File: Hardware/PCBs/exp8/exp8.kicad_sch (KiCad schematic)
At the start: 5 parts, among them J1 Conn_01x07_Female, J2 Conn_01x02_Female, U1 7410, U2 7410, U3 7400

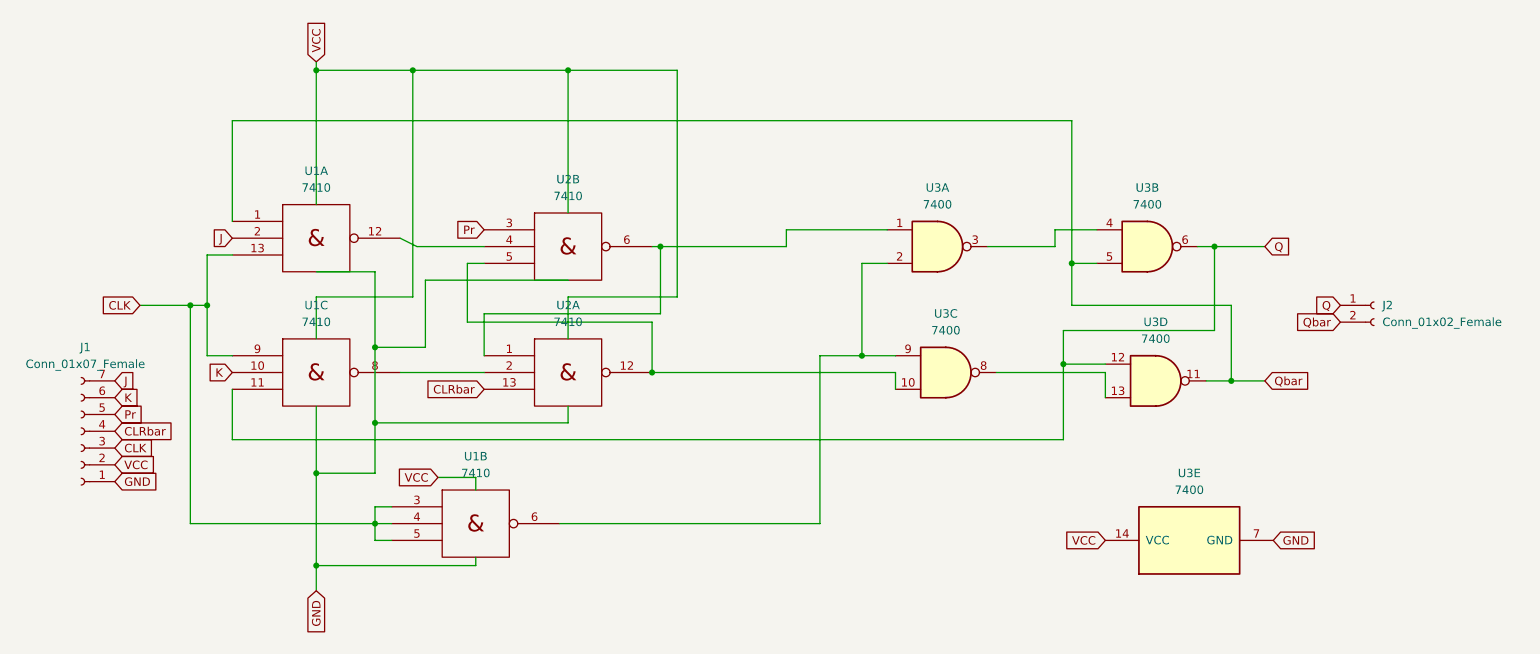
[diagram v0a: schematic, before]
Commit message: Multiple PCBs updated
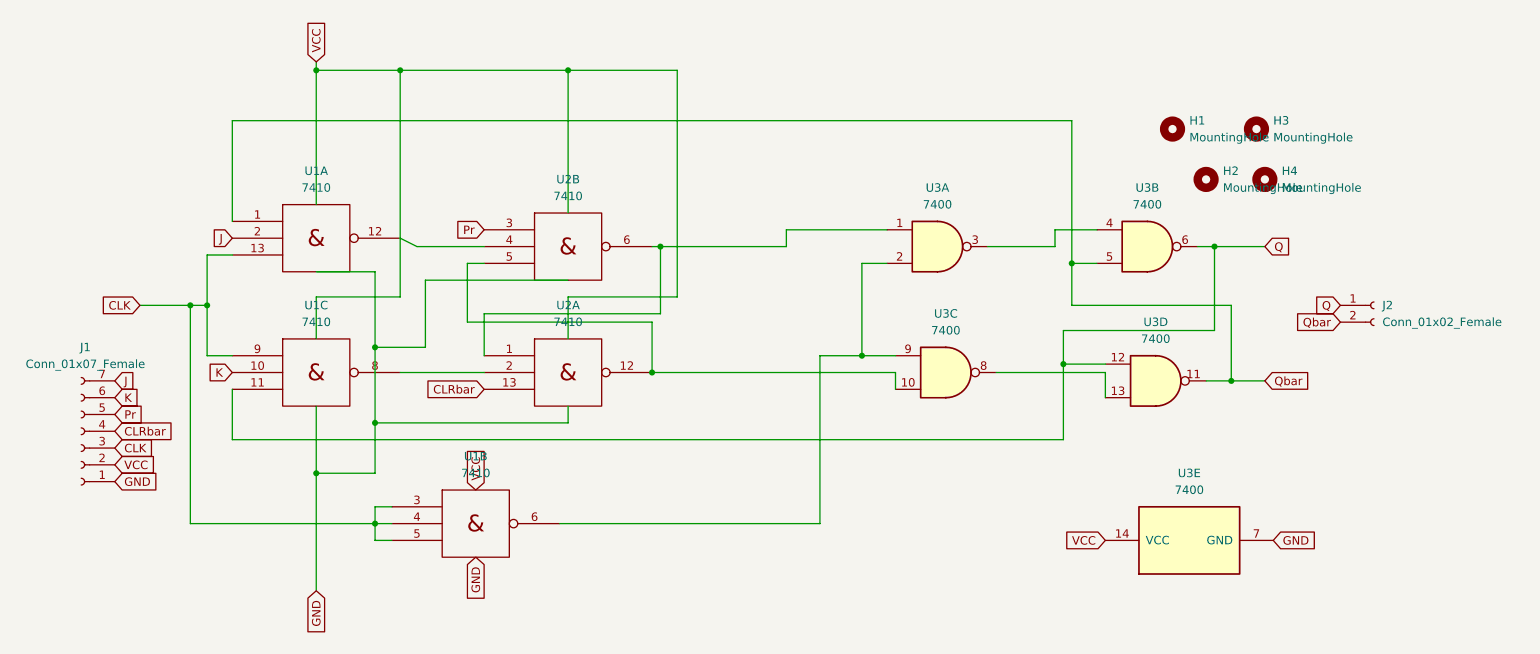
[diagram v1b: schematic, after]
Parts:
- added H1, H2, H3, H4: MountingHole, MountingHole:MountingHole_2.5mm, symbol Mechanical:MountingHole
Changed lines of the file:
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@@
   (junction (at 57.15 21.59) (diameter 0) (color 0 0 0 0)
   )
-  (junction (at 71.755 21.59) (diameter 0) (color 0 0 0 0)
-  )
   (junction (at 40.64 57.15) (diameter 0) (color 0 0 0 0)
   )
@@
   (junction (at 139.7 64.77) (diameter 0) (color 0 0 0 0)
   )
-  (junction (at 57.15 96.52) (diameter 0) (color 0 0 0 0)
-  )
   (junction (at 107.95 67.31) (diameter 0) (color 0 0 0 0)
   )
   (junction (at 171.45 50.8) (diameter 0) (color 0 0 0 0)
   )
+  (junction (at 69.85 21.59) (diameter 0) (color 0 0 0 0)
+  )
   (junction (at 95.25 21.59) (diameter 0) (color 0 0 0 0)
   )
@@
     (stroke (width 0) (type default) (color 0 0 0 0))
   )
-  (wire (pts (xy 57.15 21.59) (xy 71.755 21.59))
-    (stroke (width 0) (type default) (color 0 0 0 0))
-  )
   (wire (pts (xy 95.25 72.39) (xy 95.25 74.93))
     (stroke (width 0) (type default) (color 0 0 0 0))
@@
     (stroke (width 0) (type default) (color 0 0 0 0))
   )
-  (wire (pts (xy 95.25 21.59) (xy 71.755 21.59))
-    (stroke (width 0) (type default) (color 0 0 0 0))
-  )
-  (wire (pts (xy 57.15 55.88) (xy 71.755 55.88))
+  (wire (pts (xy 95.25 21.59) (xy 69.85 21.59))
+    (stroke (width 0) (type default) (color 0 0 0 0))
+  )
+  (wire (pts (xy 57.15 55.88) (xy 69.85 55.88))
     (stroke (width 0) (type default) (color 0 0 0 0))
   )
@@
     (stroke (width 0) (type default) (color 0 0 0 0))
   )
-  (wire (pts (xy 75.565 83.185) (xy 81.28 83.185))
-    (stroke (width 0) (type default) (color 0 0 0 0))
-  )
   (wire (pts (xy 168.91 48.26) (xy 168.91 45.72))
     (stroke (width 0) (type default) (color 0 0 0 0))
@@
     (stroke (width 0) (type default) (color 0 0 0 0))
   )
-  (wire (pts (xy 57.15 82.55) (xy 57.15 96.52))
+  (wire (pts (xy 57.15 82.55) (xy 57.15 100.33))
     (stroke (width 0) (type default) (color 0 0 0 0))
   )
@@
     (stroke (width 0) (type default) (color 0 0 0 0))
   )
-  (wire (pts (xy 57.15 96.52) (xy 57.15 100.33))
-    (stroke (width 0) (type default) (color 0 0 0 0))
-  )
   (wire (pts (xy 109.22 48.26) (xy 128.27 48.26))
     (stroke (width 0) (type default) (color 0 0 0 0))
@@
     (stroke (width 0) (type default) (color 0 0 0 0))
   )
-  (wire (pts (xy 71.755 21.59) (xy 71.755 55.88))
+  (wire (pts (xy 69.85 21.59) (xy 69.85 55.88))
     (stroke (width 0) (type default) (color 0 0 0 0))
   )
@@
     (stroke (width 0) (type default) (color 0 0 0 0))
   )
-  (wire (pts (xy 81.28 95.25) (xy 81.28 96.52))
-    (stroke (width 0) (type default) (color 0 0 0 0))
-  )
   (wire (pts (xy 66.04 74.93) (xy 66.04 82.55))
     (stroke (width 0) (type default) (color 0 0 0 0))
@@
     (stroke (width 0) (type default) (color 0 0 0 0))
   )
-  (wire (pts (xy 81.28 83.185) (xy 81.28 85.09))
-    (stroke (width 0) (type default) (color 0 0 0 0))
-  )
   (wire (pts (xy 66.04 87.63) (xy 66.04 90.17))
     (stroke (width 0) (type default) (color 0 0 0 0))
@@
     (stroke (width 0) (type default) (color 0 0 0 0))
   )
-  (wire (pts (xy 81.28 96.52) (xy 57.15 96.52))
+  (wire (pts (xy 69.85 21.59) (xy 57.15 21.59))
     (stroke (width 0) (type default) (color 0 0 0 0))
   )
@@
     )
   )
-  (global_label "VCC" (shape input) (at 75.565 83.185 180) (fields_autoplaced)
-    (effects (font (size 1.27 1.27)) (justify right))
-    (property "Intersheet References" "${INTERSHEET_REFS}" (id 0) (at 69.5233 83.1056 0)
-      (effects (font (size 1.27 1.27)) (justify right) hide)
-    )
-  )
   (global_label "Pr" (shape input) (at 82.55 45.72 180) (fields_autoplaced)
     (effects (font (size 1.27 1.27)) (justify right))
@@
     )
   )
+  (global_label "GND" (shape input) (at 81.28 95.25 270) (fields_autoplaced)
+    (effects (font (size 1.27 1.27)) (justify right))
+    (property "Intersheet References" "${INTERSHEET_REFS}" (id 0) (at 81.3594 101.5336 90)
+      (effects (font (size 1.27 1.27)) (justify right) hide)
+    )
+  )
   (global_label "CLK" (shape input) (at 26.67 78.74 0) (fields_autoplaced)
     (effects (font (size 1.27 1.27)) (justify left))
@@
     (effects (font (size 1.27 1.27)) (justify left))
     (property "Intersheet References" "${INTERSHEET_REFS}" (id 0) (at 32.9536 83.7406 0)
+      (effects (font (size 1.27 1.27)) (justify left) hide)
+    )
+  )
+  (global_label "VCC" (shape input) (at 81.28 85.09 90) (fields_autoplaced)
+    (effects (font (size 1.27 1.27)) (justify left))
+    (property "Intersheet References" "${INTERSHEET_REFS}" (id 0) (at 81.3594 79.0483 90)
       (effects (font (size 1.27 1.27)) (justify left) hide)
     )
@@
     (pin "9")
   )
+  (symbol (lib_id "Mechanical:MountingHole") (at 200.66 38.1 0) (unit 1)
+    (in_bom yes) (on_board yes) (fields_autoplaced)
+    (property "Reference" "H4" (id 0) (at 203.2 36.8299 0)
+      (effects (font (size 1.27 1.27)) (justify left))
+    )
+    (property "Value" "MountingHole" (id 1) (at 203.2 39.3699 0)
+      (effects (font (size 1.27 1.27)) (justify left))
+    )
+    (property "Footprint" "MountingHole:MountingHole_2.5mm" (id 2) (at 200.66 38.1 0)
+      (effects (font (size 1.27 1.27)) hide)
+    )
+    (property "Datasheet" "~" (id 3) (at 200.66 38.1 0)
+      (effects (font (size 1.27 1.27)) hide)
+    )
+  )
   (symbol (lib_id "74xx_IEEE:7410") (at 81.28 90.17 0) (unit 2)
     (in_bom yes) (on_board yes) (fields_autoplaced)
@@
     (pin "9")
   )
+  (symbol (lib_id "Mechanical:MountingHole") (at 199.39 30.48 0) (unit 1)
+    (in_bom yes) (on_board yes) (fields_autoplaced)
+    (property "Reference" "H3" (id 0) (at 201.93 29.2099 0)
+      (effects (font (size 1.27 1.27)) (justify left))
+    )
+    (property "Value" "MountingHole" (id 1) (at 201.93 31.7499 0)
+      (effects (font (size 1.27 1.27)) (justify left))
+    )
+    (property "Footprint" "MountingHole:MountingHole_2.5mm" (id 2) (at 199.39 30.48 0)
+      (effects (font (size 1.27 1.27)) hide)
+    )
+    (property "Datasheet" "~" (id 3) (at 199.39 30.48 0)
+      (effects (font (size 1.27 1.27)) hide)
+    )
+  )
   (symbol (lib_id "74xx_IEEE:7410") (at 57.15 67.31 0) (unit 3)
     (in_bom yes) (on_board yes) (fields_autoplaced)
@@
     (pin "9")
   )
+  (symbol (lib_id "Mechanical:MountingHole") (at 186.69 30.48 0) (unit 1)
+    (in_bom yes) (on_board yes) (fields_autoplaced)
+    (property "Reference" "H1" (id 0) (at 189.23 29.2099 0)
+      (effects (font (size 1.27 1.27)) (justify left))
+    )
+    (property "Value" "MountingHole" (id 1) (at 189.23 31.7499 0)
+      (effects (font (size 1.27 1.27)) (justify left))
+    )
+    (property "Footprint" "MountingHole:MountingHole_2.5mm" (id 2) (at 186.69 30.48 0)
+      (effects (font (size 1.27 1.27)) hide)
+    )
+    (property "Datasheet" "~" (id 3) (at 186.69 30.48 0)
+      (effects (font (size 1.27 1.27)) hide)
+    )
+  )
+  (symbol (lib_id "Mechanical:MountingHole") (at 191.77 38.1 0) (unit 1)
+    (in_bom yes) (on_board yes) (fields_autoplaced)
+    (property "Reference" "H2" (id 0) (at 194.31 36.8299 0)
+      (effects (font (size 1.27 1.27)) (justify left))
+    )
+    (property "Value" "MountingHole" (id 1) (at 194.31 39.3699 0)
+      (effects (font (size 1.27 1.27)) (justify left))
+    )
+    (property "Footprint" "MountingHole:MountingHole_2.5mm" (id 2) (at 191.77 38.1 0)
+      (effects (font (size 1.27 1.27)) hide)
+    )
+    (property "Datasheet" "~" (id 3) (at 191.77 38.1 0)
+      (effects (font (size 1.27 1.27)) hide)
+    )
+  )
   (symbol (lib_id "Connector:Conn_01x02_Female") (at 217.17 57.15 0) (unit 1)
     (in_bom yes) (on_board yes) (fields_autoplaced)
@@
   )
   (symbol_instances
+    (path "/e8dbad7f-08bc-4307-b227-743b5f751e25"
+      (reference "H1") (unit 1) (value "MountingHole") (footprint "MountingHole:MountingHole_2.5mm")
+    )
+    (path "/ef6dab83-86bf-4aba-8127-346d4bcc6ae0"
+      (reference "H2") (unit 1) (value "MountingHole") (footprint "MountingHole:MountingHole_2.5mm")
+    )
+    (path "/d43c6ed1-d232-4ca9-b1b2-324125d9a43a"
+      (reference "H3") (unit 1) (value "MountingHole") (footprint "MountingHole:MountingHole_2.5mm")
+    )
+    (path "/8f8079cd-136d-4c81-a301-fc26834d928c"
+      (reference "H4") (unit 1) (value "MountingHole") (footprint "MountingHole:MountingHole_2.5mm")
+    )
     (path "/64d1db30-7931-4980-9a73-3694b40a474f"
       (reference "J1") (unit 1) (value "Conn_01x07_Female") (footprint "Connector_JST:JST_EH_S7B-EH_1x07_P2.50mm_Horizontal")
